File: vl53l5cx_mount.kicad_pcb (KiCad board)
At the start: 2 copper layers, 12.7 x 7.9 mm, 6 parts, among them J1 Conn_01x06_MountingPin, U1 VL53L5CXV0GC/1

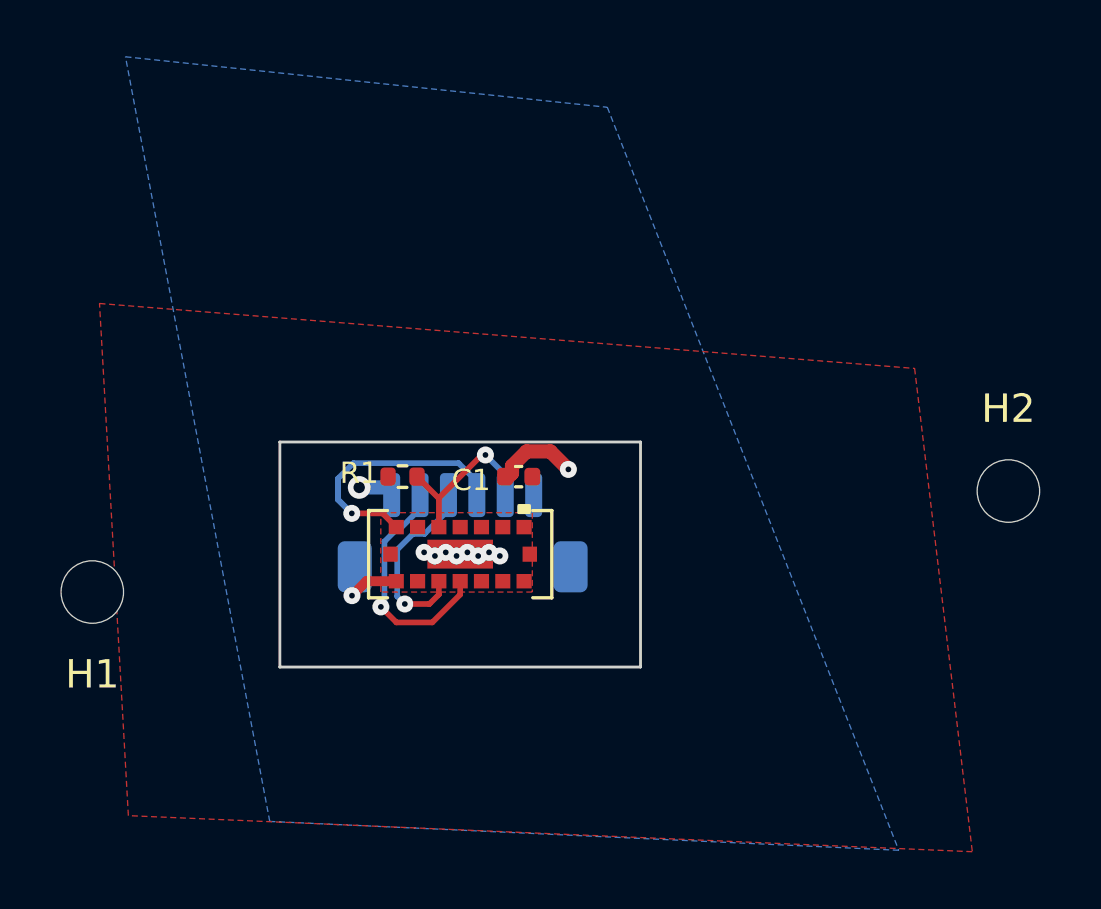
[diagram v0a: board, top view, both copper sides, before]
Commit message: clean up DRC
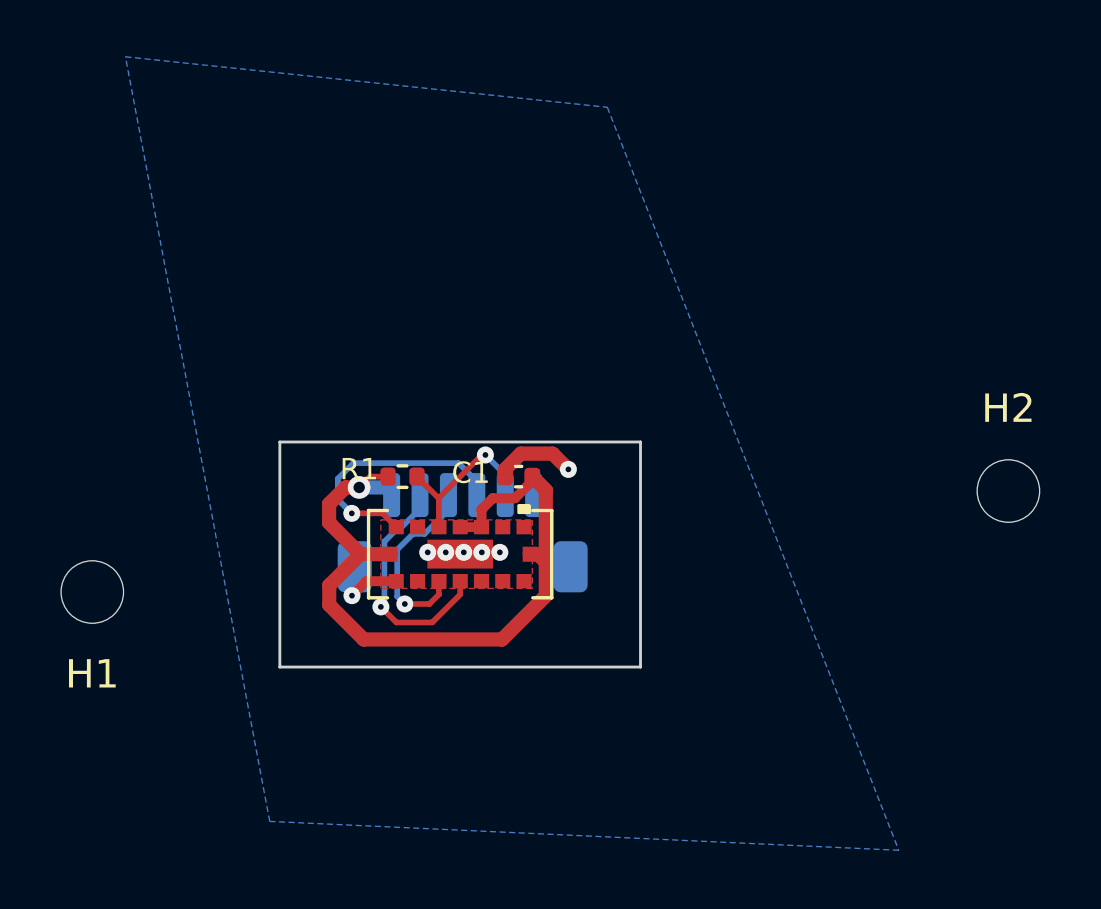
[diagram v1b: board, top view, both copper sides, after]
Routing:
- net VCC: track 1.14 -> 26.7 mm
- net Earth: track 4.65 -> 4.71 mm, vias 10 -> 7
- removed copper zone on F.Cu, net VCC
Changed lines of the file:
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@@
     (property "Sheetname" "")
     (attr smd)
-    (fp_text reference "C1" (at 1.679 -0.127 180) (layer "F.SilkS")
+    (fp_text reference "C1" (at 1.679 0.127 180) (layer "F.SilkS")
       (effects (font (size 0.75 0.75) (thickness 0.1)))
     )
@@
     (property "Sheetname" "")
     (attr smd)
-    (fp_text reference "R1" (at 1.526 0.127) (layer "F.SilkS")
+    (fp_text reference "R1" (at 1.526 0.254) (layer "F.SilkS")
       (effects (font (size 0.75 0.75) (thickness 0.1)))
     )
@@
   (gr_line (start 118.11 32.3596) (end 118.11 24.4348) (layer "Edge.Cuts") (width 0.1))
   (gr_line (start 118.11 24.4348) (end 130.81 24.4348) (layer "Edge.Cuts") (width 0.1))
+  (segment (start 120.949001 28.3845) (end 119.850489 29.483012) (width 0.5) (layer "F.Cu") (net 1))
+  (segment (start 121.062776 31.388456) (end 125.932756 31.388456) (width 0.5) (layer "F.Cu") (net 1))
+  (segment (start 125.210001 26.812277) (end 125.606278 26.416) (width 0.35) (layer "F.Cu") (net 1))
+  (segment (start 126.386351 26.416) (end 127 25.802351) (width 0.35) (layer "F.Cu") (net 1))
+  (segment (start 125.210001 27.432) (end 124.46 27.432) (width 0.35) (layer "F.Cu") (net 1))
+  (segment (start 120.425441 26.035) (end 120.904 26.035) (width 0.5) (layer "F.Cu") (net 1))
+  (segment (start 119.850489 30.176169) (end 121.062776 31.388456) (width 0.5) (layer "F.Cu") (net 1))
+  (segment (start 120.949001 28.3845) (end 119.84364 27.279139) (width 0.5) (layer "F.Cu") (net 1))
+  (segment (start 127.476212 28.670212) (end 127.1905 28.3845) (width 0.5) (layer "F.Cu") (net 1))
+  (segment (start 127 25.654) (end 127.476212 26.130212) (width 0.5) (layer "F.Cu") (net 1))
+  (segment (start 125.606278 26.416) (end 126.386351 26.416) (width 0.35) (layer "F.Cu") (net 1))
+  (segment (start 119.84364 26.616801) (end 120.425441 26.035) (width 0.5) (layer "F.Cu") (net 1))
+  (segment (start 122.0089 28.3845) (end 120.949001 28.3845) (width 0.5) (layer "F.Cu") (net 1))
+  (segment (start 127.476212 26.130212) (end 127.476212 28.670212) (width 0.5) (layer "F.Cu") (net 1))
+  (segment (start 119.850489 29.483012) (end 119.850489 30.176169) (width 0.5) (layer "F.Cu") (net 1))
+  (segment (start 125.210001 27.432) (end 125.210001 26.812277) (width 0.35) (layer "F.Cu") (net 1))
+  (segment (start 121.285 25.654) (end 120.904 26.035) (width 0.2) (layer "F.Cu") (net 1))
+  (segment (start 127 25.802351) (end 127 25.654) (width 0.35) (layer "F.Cu") (net 1))
+  (segment (start 121.92 25.654) (end 121.285 25.654) (width 0.2) (layer "F.Cu") (net 1))
+  (segment (start 119.84364 27.279139) (end 119.84364 26.616801) (width 0.5) (layer "F.Cu") (net 1))
+  (segment (start 127.1905 28.3845) (end 126.9111 28.3845) (width 0.5) (layer "F.Cu") (net 1))
+  (segment (start 125.932756 31.388456) (end 127.476212 29.845) (width 0.5) (layer "F.Cu") (net 1))
+  (segment (start 127.476212 29.845) (end 127.476212 28.670212) (width 0.5) (layer "F.Cu") (net 1))
   (via (at 120.904 26.035) (size 0.8) (drill 0.4) (layers "F.Cu" "B.Cu") (net 1))
   (segment (start 122.047 26.035) (end 120.904 26.035) (width 0.5) (layer "B.Cu") (net 1))
-  (segment (start 126.283972 25.282611) (end 126.801583 24.765) (width 0.5) (layer "F.Cu") (net 2))
-  (segment (start 127.635 24.765) (end 128.27 25.4) (width 0.5) (layer "F.Cu") (net 2))
   (segment (start 122.209999 29.337) (end 121.158 29.337) (width 0.35) (layer "F.Cu") (net 2))
-  (segment (start 126.283972 25.537028) (end 126.283972 25.282611) (width 0.5) (layer "F.Cu") (net 2))
-  (segment (start 126.801583 24.765) (end 127.635 24.765) (width 0.5) (layer "F.Cu") (net 2))
+  (segment (start 126.04 25.654) (end 126.04 25.399583) (width 0.5) (layer "F.Cu") (net 2))
+  (segment (start 126.595103 24.84448) (end 127.71448 24.84448) (width 0.5) (layer "F.Cu") (net 2))
+  (segment (start 126.04 25.399583) (end 126.595103 24.84448) (width 0.5) (layer "F.Cu") (net 2))
   (segment (start 121.158 29.337) (end 120.65 29.845) (width 0.35) (layer "F.Cu") (net 2))
-  (segment (start 126.167 25.654) (end 126.283972 25.537028) (width 0.5) (layer "F.Cu") (net 2))
-  (via (at 125.476 28.321) (size 0.6) (drill 0.2) (layers "F.Cu" "B.Cu") (net 2))
-  (via (at 125.857 28.448) (size 0.6) (drill 0.2) (layers "F.Cu" "B.Cu") (free) (net 2))
-  (via (at 123.19 28.321) (size 0.6) (drill 0.2) (layers "F.Cu" "B.Cu") (free) (net 2))
+  (segment (start 127.71448 24.84448) (end 128.27 25.4) (width 0.5) (layer "F.Cu") (net 2))
+  (via (at 125.857 28.321) (size 0.6) (drill 0.2) (layers "F.Cu" "B.Cu") (free) (net 2))
+  (via (at 125.222 28.321) (size 0.6) (drill 0.2) (layers "F.Cu" "B.Cu") (net 2))
+  (via (at 123.317 28.321) (size 0.6) (drill 0.2) (layers "F.Cu" "B.Cu") (free) (net 2))
   (via (at 120.65 29.845) (size 0.6) (drill 0.2) (layers "F.Cu" "B.Cu") (net 2))
-  (via (at 124.714 28.321) (size 0.6) (drill 0.2) (layers "F.Cu" "B.Cu") (net 2))
+  (via (at 124.587 28.321) (size 0.6) (drill 0.2) (layers "F.Cu" "B.Cu") (net 2))
   (via (at 123.952 28.321) (size 0.6) (drill 0.2) (layers "F.Cu" "B.Cu") (net 2))
-  (via (at 125.095 28.448) (size 0.6) (drill 0.2) (layers "F.Cu" "B.Cu") (net 2))
   (via (at 128.27 25.4) (size 0.6) (drill 0.2) (layers "F.Cu" "B.Cu") (net 2))
-  (via (at 123.571 28.448) (size 0.6) (drill 0.2) (layers "F.Cu" "B.Cu") (net 2))
-  (via (at 124.333 28.448) (size 0.6) (drill 0.2) (layers "F.Cu" "B.Cu") (net 2))
   (segment (start 122.21551 30.788936) (end 123.477785 30.788936) (width 0.2) (layer "F.Cu") (net 3))
   (segment (start 121.667683 30.241109) (end 122.21551 30.788936) (width 0.2) (layer "F.Cu") (net 3))
@@
   (segment (start 126.047 26.304) (end 126.047 25.59) (width 0.2) (layer "B.Cu") (net 7))
   (segment (start 126.047 25.59) (end 125.349 24.892) (width 0.2) (layer "B.Cu") (net 7))
-  (zone (net 1) (net_name "VCC") (layer "F.Cu") (hatch edge 0.508)
-    (connect_pads (clearance 0.3))
-    (min_thickness 0.254) (filled_areas_thickness no)
-    (fill yes (thermal_gap 0.508) (thermal_bridge_width 0.3))
-    (polygon
-      (pts
-        (xy 140.462 21.844)
-        (xy 142.494 38.862)
-        (xy 112.776 37.592)
-        (xy 111.76 19.558)
-      )
-    )
-  )
   (zone (net 2) (net_name "Earth") (layer "F.Cu") (hatch edge 0.508)
     (connect_pads yes (clearance 0.3))
@@
     (polygon
       (pts
-        (xy 127 29.718)
-        (xy 121.666 29.718)
-        (xy 121.666 26.924)
-        (xy 127 26.924)
+        (xy 127 29.591)
+        (xy 121.666 29.591)
+        (xy 121.666 27.178)
+        (xy 127 27.178)
       )
     )
